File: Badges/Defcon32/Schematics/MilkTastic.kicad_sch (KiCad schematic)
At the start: 3 parts, among them U1 MilkV Duo

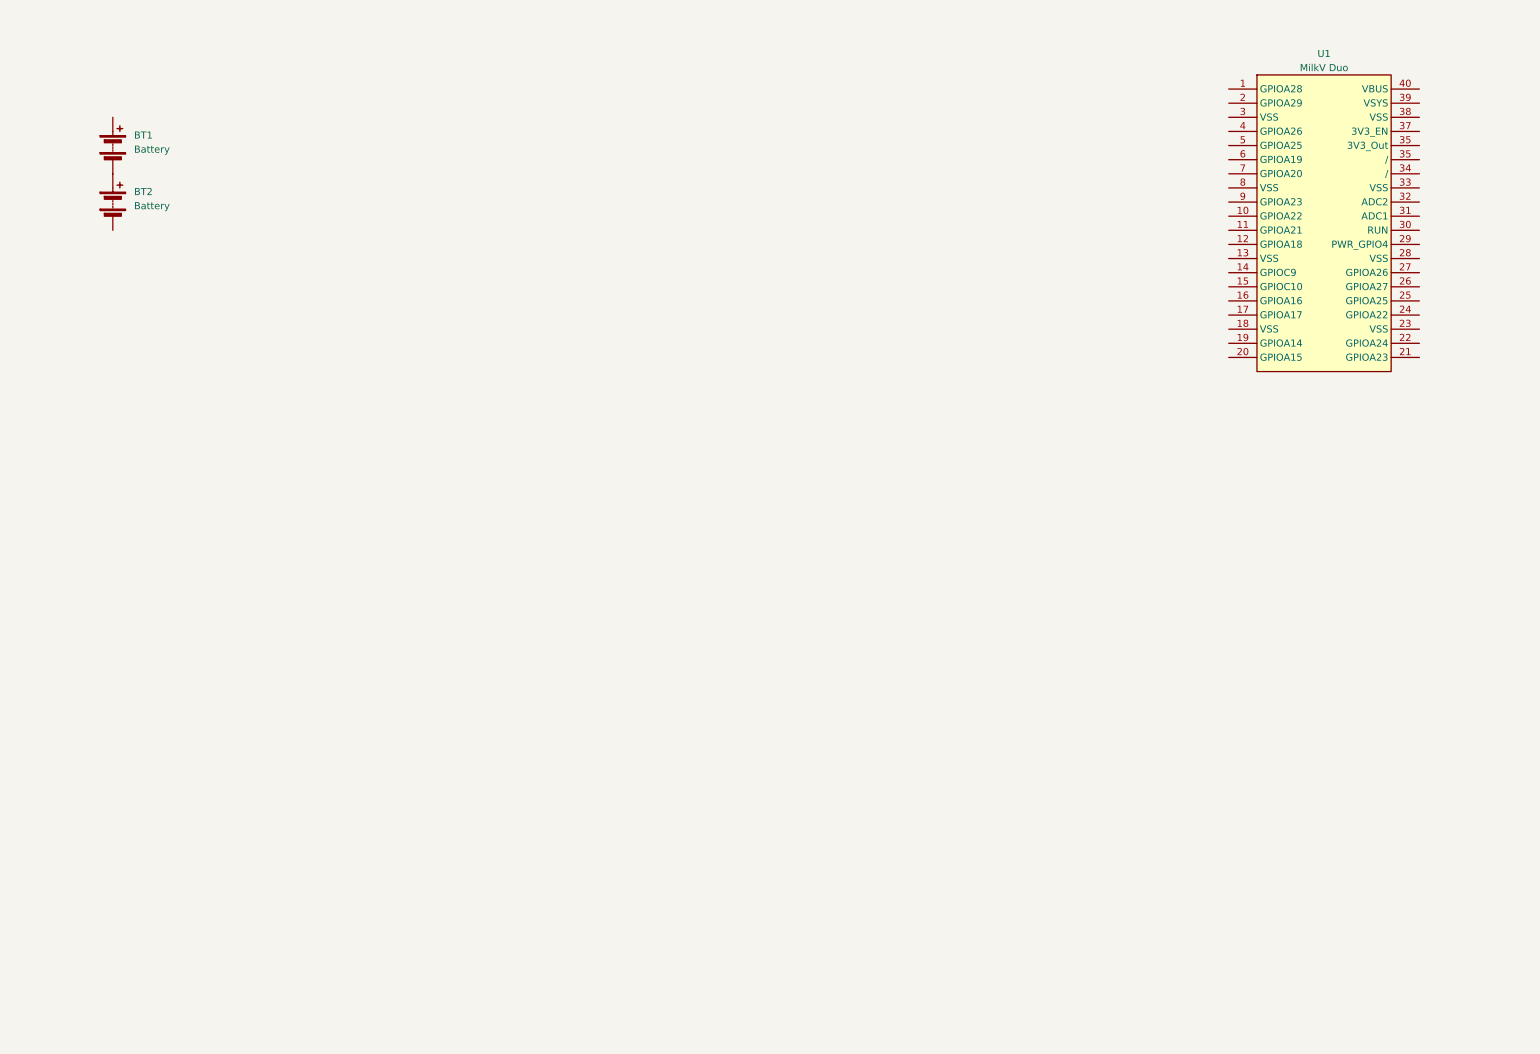
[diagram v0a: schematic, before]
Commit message: Ready to start PCB
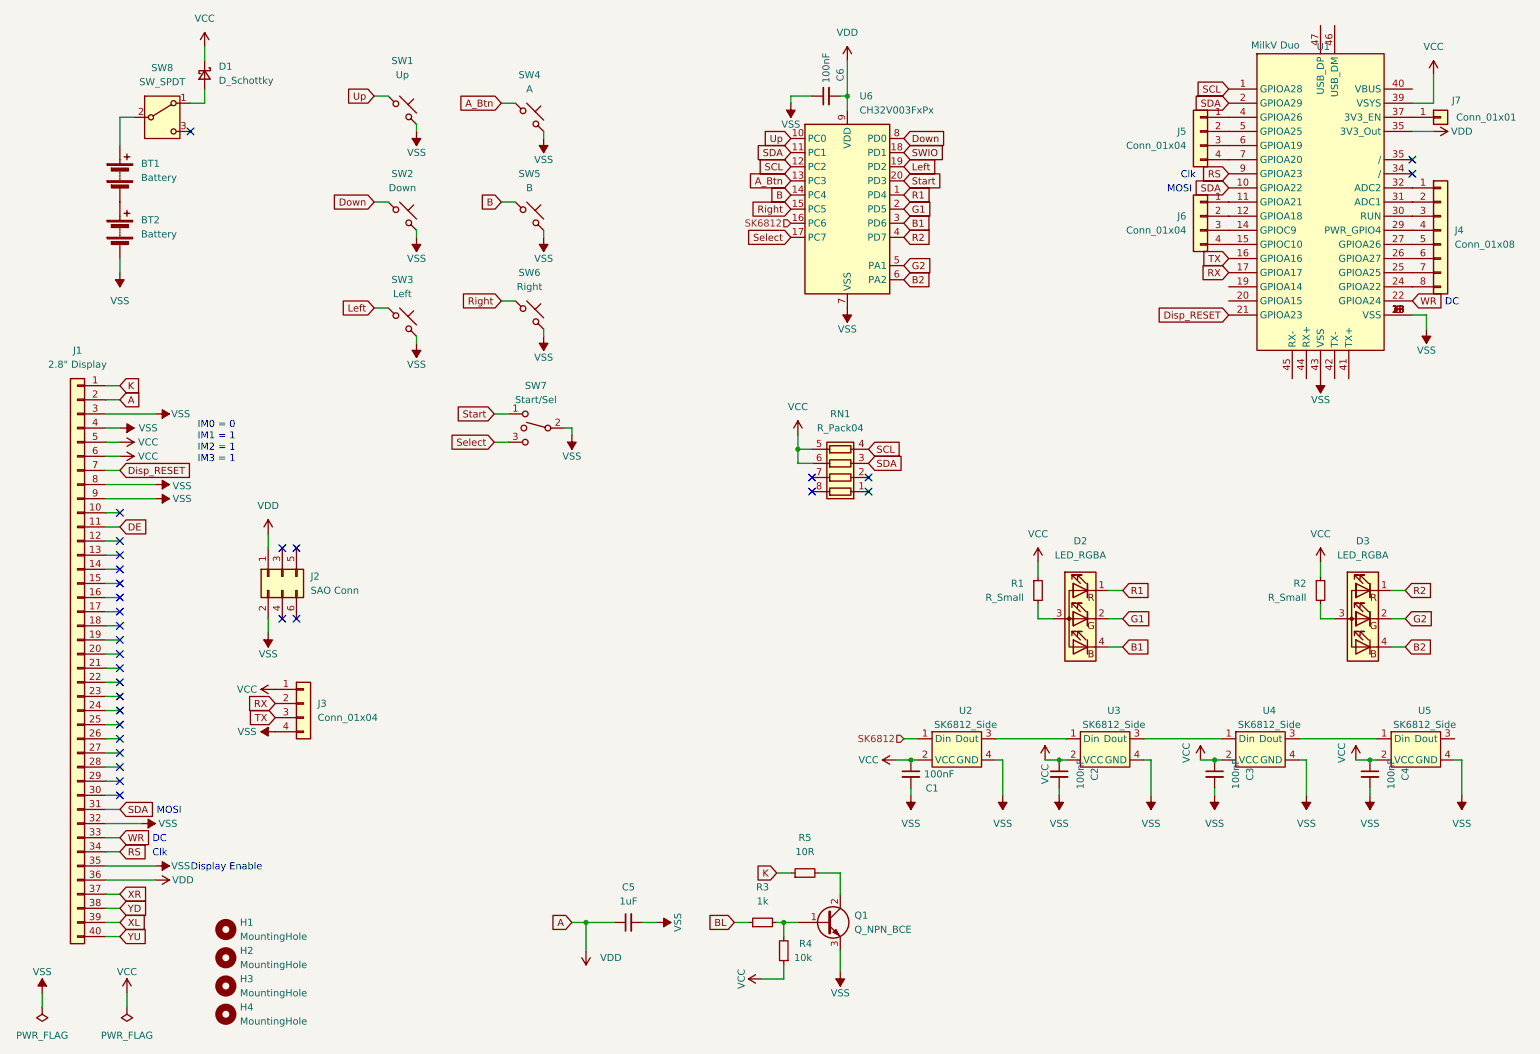
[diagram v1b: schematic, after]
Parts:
- added C1, C2, C3, C4, C6: 100nF, Capacitor_SMD:C_0805_2012Metric, symbol Device:C_Small
- added C5: 1uF, Capacitor_SMD:C_0805_2012Metric, symbol Device:C_Small
- added D1: D_Schottky, Diode_SMD:D_0805_2012Metric, symbol Device:D_Schottky_Small
- added D2, D3: LED_RGBA, UL_LED:XL-3227RGB_LED, symbol Device:LED_RGBA
- added H1, H2, H3, H4: MountingHole, MountingHole:MountingHole_3.2mm_M3, symbol Mechanical:MountingHole
- added J1: 2.8" Display, UE-Connector:Omron_XF2M-4015-1A_1x40-1MP_P0.5mm_Horizontal, symbol Connector_Generic:Conn_01x40
- added J2: SAO Conn, Connector_PinSocket_2.54mm:PinSocket_2x03_P2.54mm_Vertical, symbol Connector_Generic:Conn_02x03_Odd_Even
- added J3, J5, J6: Conn_01x04, Connector_PinHeader_2.54mm:PinHeader_1x04_P2.54mm_Vertical, symbol Connector_Generic:Conn_01x04
- added J4: Conn_01x08, Connector_PinHeader_2.54mm:PinHeader_1x08_P2.54mm_Vertical, symbol Connector_Generic:Conn_01x08
- added J7: Conn_01x01, Connector_PinHeader_2.54mm:PinHeader_1x01_P2.54mm_Vertical, symbol Connector_Generic:Conn_01x01
- added Q1: Q_NPN_BCE, Package_TO_SOT_SMD:SOT-23, symbol Device:Q_NPN_BCE
- added R1, R2: R_Small, Resistor_SMD:R_0805_2012Metric, symbol Device:R_Small
- added R3: 1k, Resistor_SMD:R_0805_2012Metric, symbol Device:R_Small
- added R4: 10k, Resistor_SMD:R_0805_2012Metric, symbol Device:R_Small
- added R5: 10R, Resistor_SMD:R_0805_2012Metric, symbol Device:R_Small
- added RN1: R_Pack04, Resistor_SMD:R_Array_Convex_4x0603, symbol Device:R_Pack04
- added SW1: Up, UL_Buttons:BZCN-TSC005A_Button, symbol Switch:SW_Push_45deg
- added SW2: Down, UL_Buttons:BZCN-TSC005A_Button, symbol Switch:SW_Push_45deg
- added SW3: Left, UL_Buttons:BZCN-TSC005A_Button, symbol Switch:SW_Push_45deg
- added SW4: A, UL_Buttons:BZCN-TSC005A_Button, symbol Switch:SW_Push_45deg
- added SW5: B, UL_Buttons:BZCN-TSC005A_Button, symbol Switch:SW_Push_45deg
- added SW6: Right, UL_Buttons:BZCN-TSC005A_Button, symbol Switch:SW_Push_45deg
- added SW7: Start/Sel, UL_Buttons:StartSel, symbol Switch:SW_SPDT_MSM
- added SW8: SW_SPDT, UL_Buttons:SK-3296S_switch, symbol Switch:SW_SPDT
- added U2, U3, U4, U5: SK6812_Side, UL_LED:SK6812SIDE-A-RVS, symbol BSides22:SK6812_Side
- added U6: CH32V003FxPx, Package_SO:TSSOP-20_4.4x6.5mm_P0.65mm, symbol MCU_WCH_CH32V0:CH32V003FxPx
- BT1, BT2: footprint (none) -> UE-Battery:AA_TH
- U1: footprint (none) -> UL_Module:MIlkV-Duo
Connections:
- net VSS: now reaches BT2.2 (-)
- net VSS: now also U1.13 (VSS), U1.18 (VSS), U1.23 (VSS), U1.28 (VSS), U1.3 (VSS), U1.33 (VSS), U1.38 (VSS), U1.43 (VSS), U1.8 (VSS), C1.2, C2.2, C3.2, C4.2, C5.2, C6.1, J1.3 (Pin_3), J1.32 (Pin_32), J1.35 (Pin_35), J1.4 (Pin_4), J1.8 (Pin_8), J1.9 (Pin_9), J2.2 (Pin_2), J3.4 (Pin_4), Q1.3 (E), SW1.2, SW2.2, SW3.2, SW4.2, SW5.2, SW6.2, SW7.2, U2.4 (GND), U3.4 (GND), U4.4 (GND), U5.4 (GND), U6.7 (VSS)
- net at BT1.1 (+): now also SW8.2 (B)
- net SCL: now reaches U1.1 (GPIOA28)
- net SCL: now also RN1.4 (R4.1), U6.12 (PC2)
- net SDA: now reaches U1.10 (GPIOA22)
- net SDA: now also U1.2 (GPIOA29), J1.31 (Pin_31), RN1.3 (R3.1), U6.11 (PC1)
- net at U1.11 (GPIOA21): now also J6.1 (Pin_1)
- net at U1.12 (GPIOA18): now also J6.2 (Pin_2)
- net at U1.14 (GPIOC9): now also J6.3 (Pin_3)
- net at U1.15 (GPIOC10): now also J6.4 (Pin_4)
- net TX: now reaches U1.16 (GPIOA16)
- net TX: now also J3.3 (Pin_3)
- net RX: now reaches U1.17 (GPIOA17)
- net RX: now also J3.2 (Pin_2)
- net Disp_RESET: now reaches U1.21 (GPIOA23)
- net Disp_RESET: now also J1.7 (Pin_7)
- net WR: now reaches U1.22 (GPIOA24)
- net WR: now also J1.33 (Pin_33)
- net at U1.24 (GPIOA22): now also J4.8 (Pin_8)
- net at U1.25 (GPIOA25): now also J4.7 (Pin_7)
- net at U1.26 (GPIOA27): now also J4.6 (Pin_6)
- net at U1.27 (GPIOA26): now also J4.5 (Pin_5)
- net at U1.29 (PWR_GPIO4): now also J4.4 (Pin_4)
- net at U1.30 (RUN): now also J4.3 (Pin_3)
- net at U1.31 (ADC1): now also J4.2 (Pin_2)
- net at U1.32 (ADC2): now also J4.1 (Pin_1)
- net VDD: now reaches U1.35 (3V3_Out)
- net VDD: now also C5.1, C6.2, J1.2 (Pin_2), J1.36 (Pin_36), J2.1 (Pin_1), U6.9 (VDD)
- net at U1.37 (3V3_EN): now also J7.1 (Pin_1)
- net VCC: now reaches U1.39 (VSYS)
- net VCC: now also C1.1, C2.1, C3.1, C4.1, D1.1 (K), J1.5 (Pin_5), J1.6 (Pin_6), J3.1 (Pin_1), R1.1, R2.1, R4.1, RN1.5 (R4.2), RN1.6 (R3.2), U2.2 (VCC), U3.2 (VCC), U4.2 (VCC), U5.2 (VCC)
- net at U1.4 (GPIOA26): now also J5.1 (Pin_1)
- net at U1.5 (GPIOA25): now also J5.2 (Pin_2)
- net at U1.6 (GPIOA19): now also J5.3 (Pin_3)
- net at U1.7 (GPIOA20): now also J5.4 (Pin_4)
- net RS: now reaches U1.9 (GPIOA23)
- net RS: now also J1.34 (Pin_34)
- new net: U2.3 (Dout), U3.1 (Din)
- new net: D2.3 (A), R1.2
- new net: U4.3 (Dout), U5.1 (Din)
- new net: Q1.1 (B), R3.2, R4.2
- new net: U3.3 (Dout), U4.1 (Din)
- new net: Q1.2 (C), R5.2
- new net: D3.3 (A), R2.2
- new net: D1.2 (A), SW8.1 (A)
- new net A_Btn: SW4.1, U6.13 (PC3)
- new net B: SW5.1, U6.14 (PC4)
- new net B1: D2.4 (BK), U6.3 (PD6)
- new net B2: D3.4 (BK), U6.6 (PA2)
- new net BL: R3.1
- new net DE: J1.11 (Pin_11)
- new net Down: SW2.1, U6.8 (PD0)
- new net G1: D2.2 (GK), U6.2 (PD5)
- new net G2: D3.2 (GK), U6.5 (PA1)
- new net K: J1.1 (Pin_1), R5.1
- new net Left: SW3.1, U6.19 (PD2)
- new net R1: D2.1 (RK), U6.1 (PD4)
- new net R2: D3.1 (RK), U6.4 (PD7)
- new net Right: SW6.1, U6.15 (PC5)
- new net SK6812: U2.1 (Din), U6.16 (PC6)
- new net SWIO: U6.18 (PD1)
- new net Select: SW7.3, U6.17 (PC7)
- new net Start: SW7.1, U6.20 (PD3)
- new net Up: SW1.1, U6.10 (PC0)
- new net XL: J1.39 (Pin_39)
- new net XR: J1.37 (Pin_37)
- new net YD: J1.38 (Pin_38)
- new net YU: J1.40 (Pin_40)
- no-connect marks 0 -> 31
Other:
- note added: "Clk"
- note added: "DC"
- note added: "Display Enable"
- note added: "IM0 = 0 IM1 = 1 IM2 = 1 IM3 = 1"
- note added: "MOSI"
- moved on the sheet: BT1, BT2

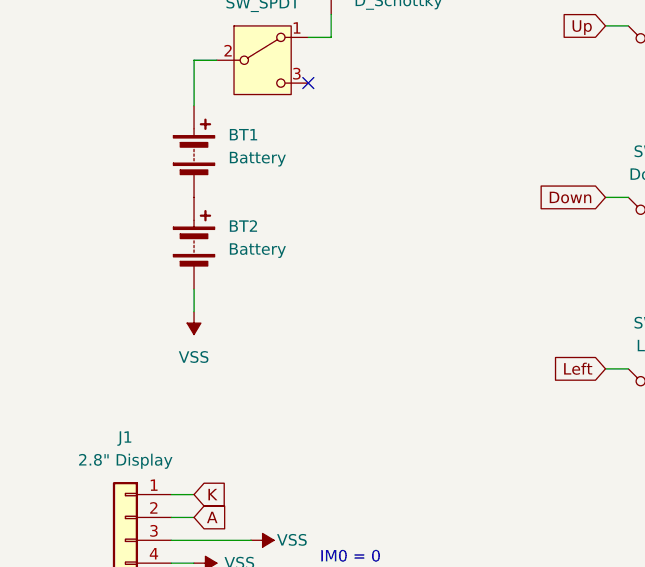
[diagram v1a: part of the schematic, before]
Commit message: Some Schematic
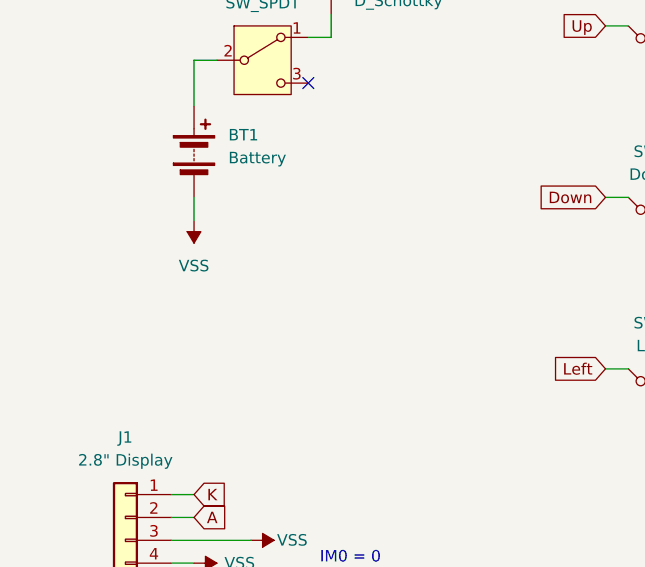
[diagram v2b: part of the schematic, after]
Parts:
- removed BT2: Battery, UE-Battery:AA_TH, symbol Device:Battery
- BT1: footprint UE-Battery:AA_TH -> UE-Battery:AAA_TH_UM-4
- D2, D3: footprint UL_LED:XL-3227RGB_LED -> UE_LED:XL-3227RGB_LED
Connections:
- net VSS: now also BT1.2 (-)
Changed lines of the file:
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@@
 	(wire
 		(pts
-			(xy 31.75 57.15) (xy 31.75 59.69)
+			(xy 31.75 46.99) (xy 31.75 49.53)
 		)
 		(stroke
@@
 	)
 	(symbol
-		(lib_id "Device:Battery")
-		(at 31.75 52.07 0)
-		(unit 1)
-		(exclude_from_sim no)
-		(in_bom yes)
-		(on_board yes)
-		(dnp no)
-		(fields_autoplaced yes)
-		(property "Reference" "BT2"
-			(at 35.56 50.2284 0)
-			(effects
-				(font
-					(size 1.27 1.27)
-				)
-				(justify left)
-			)
-		)
-		(property "Value" "Battery"
-			(at 35.56 52.7684 0)
-			(effects
-				(font
-					(size 1.27 1.27)
-				)
-				(justify left)
-			)
-		)
-		(property "Footprint" "UE-Battery:AA_TH"
-			(at 31.75 50.546 90)
-			(effects
-				(font
-					(size 1.27 1.27)
-				)
-				(hide yes)
-			)
-		)
-		(property "Datasheet" "~"
-			(at 31.75 50.546 90)
-			(effects
-				(font
-					(size 1.27 1.27)
-				)
-				(hide yes)
-			)
-		)
-		(property "Description" "Multiple-cell battery"
-			(at 31.75 52.07 0)
-			(effects
-				(font
-					(size 1.27 1.27)
-				)
-				(hide yes)
-			)
-		)
-		(pin "1"
-		)
-		(pin "2"
-		)
-		(instances
-			(project "MilkTastic"
-				(path "/625bbc85-a8f8-46d4-9338-e60d5e5e321d"
-					(reference "BT2")
-					(unit 1)
-				)
-			)
-		)
-	)
-	(symbol
 		(lib_id "power:VSS")
 		(at 17.78 189.23 0)
@@
 			)
 		)
-		(property "Footprint" "UL_LED:XL-3227RGB_LED"
+		(property "Footprint" "UE_LED:XL-3227RGB_LED"
 			(at 204.47 132.08 0)
 			(effects
@@
 	(symbol
 		(lib_id "power:VSS")
-		(at 31.75 59.69 180)
+		(at 31.75 49.53 180)
 		(unit 1)
 		(exclude_from_sim no)
@@
 		(fields_autoplaced yes)
 		(property "Reference" "#PWR01"
-			(at 31.75 55.88 0)
+			(at 31.75 45.72 0)
 			(effects
 				(font
@@
 		)
 		(property "Value" "VSS"
-			(at 31.75 64.77 0)
+			(at 31.75 54.61 0)
 			(effects
 				(font
@@
 		)
 		(property "Footprint" ""
-			(at 31.75 59.69 0)
+			(at 31.75 49.53 0)
 			(effects
 				(font
@@
 		)
 		(property "Datasheet" ""
-			(at 31.75 59.69 0)
+			(at 31.75 49.53 0)
 			(effects
 				(font
@@
 		)
 		(property "Description" "Power symbol creates a global label with name \"VSS\""
-			(at 31.75 59.69 0)
+			(at 31.75 49.53 0)
 			(effects
 				(font
@@
 			)
 		)
-		(property "Footprint" "UE-Battery:AA_TH"
+		(property "Footprint" "UE-Battery:AAA_TH_UM-4"
 			(at 31.75 40.386 90)
 			(effects
@@
 			)
 		)
-		(property "Footprint" "UL_LED:XL-3227RGB_LED"
+		(property "Footprint" "UE_LED:XL-3227RGB_LED"
 			(at 255.27 132.08 0)
 			(effects
